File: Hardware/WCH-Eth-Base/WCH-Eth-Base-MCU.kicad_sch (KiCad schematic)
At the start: 47 parts, among them J1 Conn_02x03_Odd_Even, J2 Micro_SD_Card_Det1, J3 USB_C_Receptacle_USB2.0, J4 USB_C_Receptacle_USB2.0, SW1 SW_Push, SW2 SW_Push, U1 CH32V307VCT6, U2 WE-TVS-82400102, U3 WE-TVS-82400102, Y1 Crystal_GND24

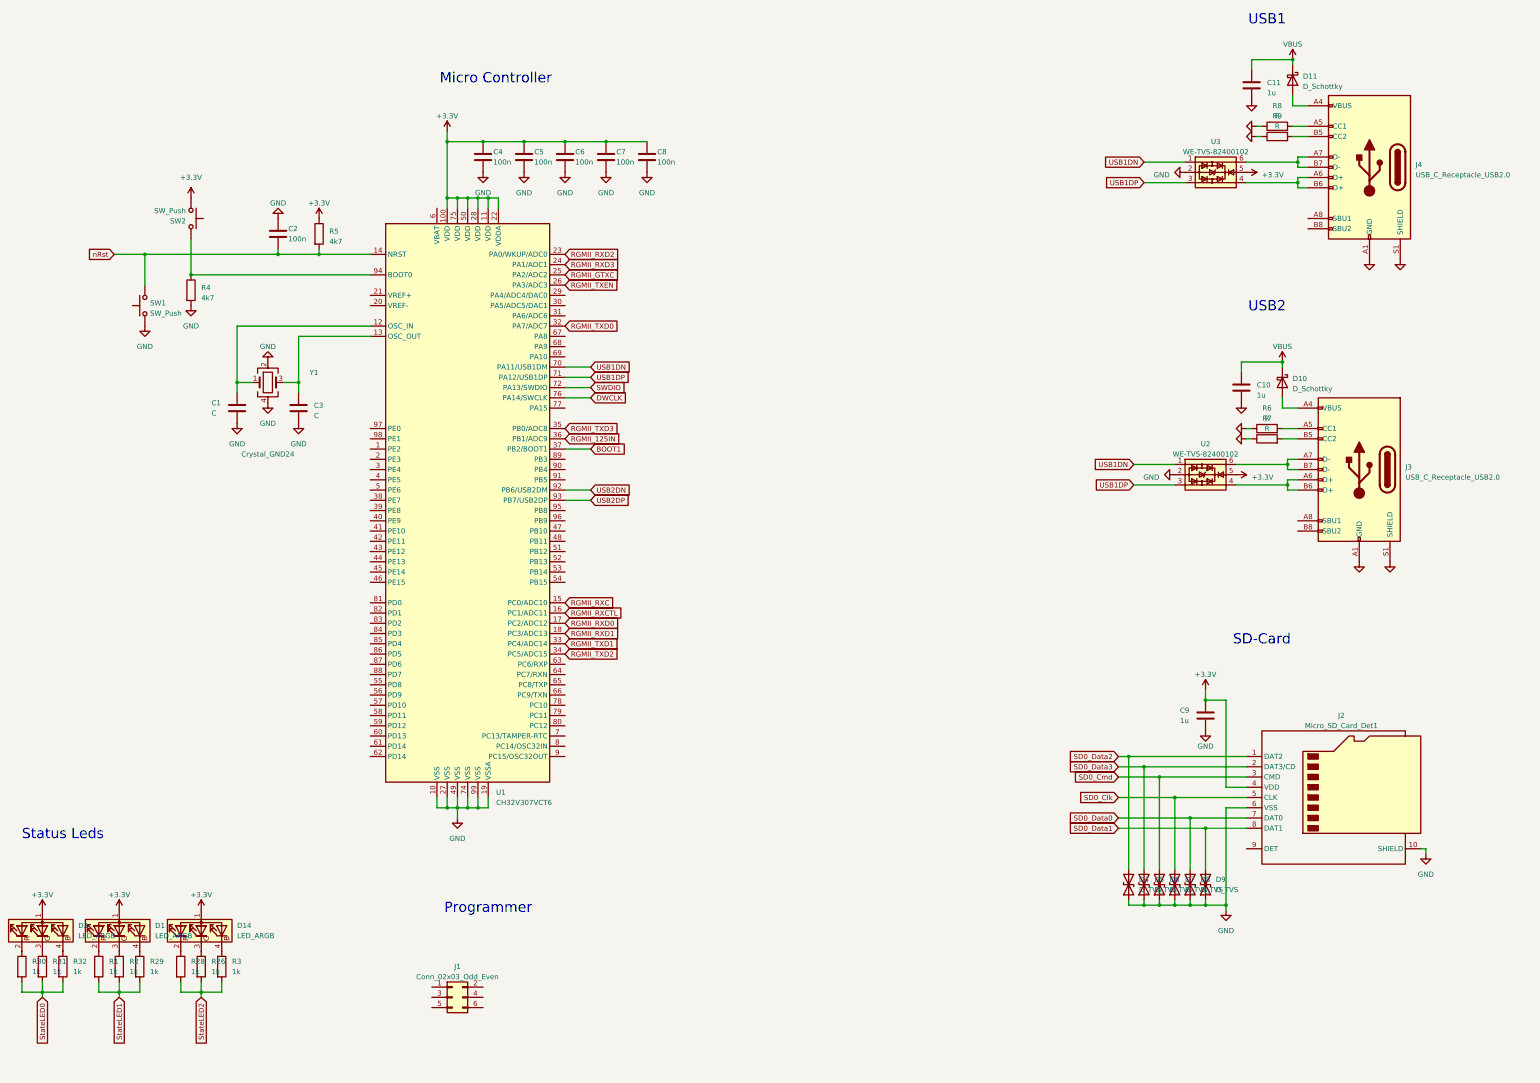
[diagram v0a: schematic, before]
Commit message: add Files and First Layout things
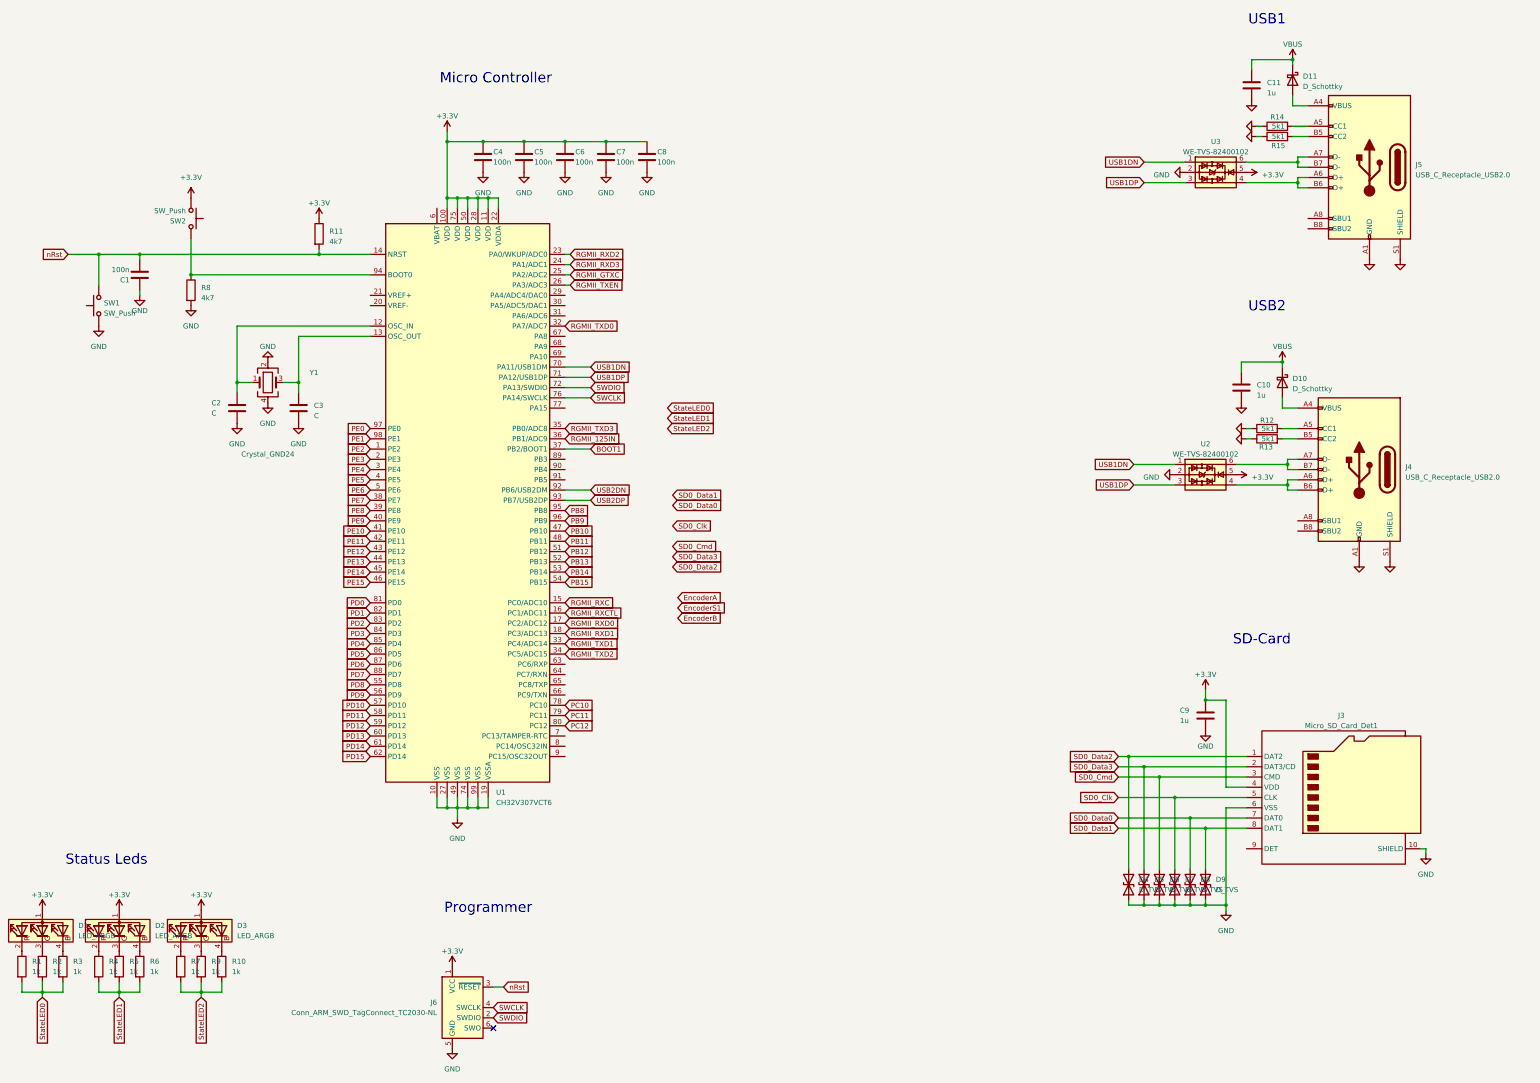
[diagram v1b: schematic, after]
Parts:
- removed J1: Conn_02x03_Odd_Even, symbol Connector_Generic:Conn_02x03_Odd_Even
- added J6: Conn_ARM_SWD_TagConnect_TC2030-NL, Connector:Tag-Connect_TC2030-IDC-NL_2x03_P1.27mm_Vertical, symbol Connector:Conn_ARM_SWD_TagConnect_TC2030-NL
- D10, D11, D4: footprint (none) -> Diode_SMD:D_SMA
- R12: renamed from R6; value R -> 5k1
- R13: renamed from R7; value R -> 5k1
- R14: renamed from R8; value R -> 5k1
- R15: renamed from R9; value R -> 5k1
- SW1, SW2: footprint (none) -> LCSC:SW-SMD_4P-L5.1-W5.1-P3.70-LS6.5-TL-2
- renumbered C2 to C1, C1 to C2, D2 to D1, D1 to D2, D14 to D3, J2 to J3, J3 to J4, J4 to J5, R30 to R1, R3 to R10, R5 to R11, R31 to R2, R32 to R3, R1 to R4, R2 to R5, R29 to R6, R28 to R7, R4 to R8, R26 to R9
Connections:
- net +3.3V: now also J6.1 (VCC)
- net GND: now also J6.5 (GND)
- net SWDIO: now also J6.2 (SWDIO)
- net nRst: now also J6.3 (~{RESET})
- net PE2: now reaches U1.1 (PE2)
- net PE3: now reaches U1.2 (PE3)
- net PE4: now reaches U1.3 (PE4)
- net PE7: now reaches U1.38 (PE7)
- net PE8: now reaches U1.39 (PE8)
- net PE5: now reaches U1.4 (PE5)
- net PE9: now reaches U1.40 (PE9)
- net PE10: now reaches U1.41 (PE10)
- net PE11: now reaches U1.42 (PE11)
- net PE12: now reaches U1.43 (PE12)
- net PE13: now reaches U1.44 (PE13)
- net PE14: now reaches U1.45 (PE14)
- net PE15: now reaches U1.46 (PE15)
- net PB10: now reaches U1.47 (PB10)
- net PB11: now reaches U1.48 (PB11)
- net PE6: now reaches U1.5 (PE6)
- net PB12: now reaches U1.51 (PB12)
- net PB13: now reaches U1.52 (PB13)
- net PB14: now reaches U1.53 (PB14)
- net PB15: now reaches U1.54 (PB15)
- net PD8: now reaches U1.55 (PD8)
- net PD9: now reaches U1.56 (PD9)
- net PD10: now reaches U1.57 (PD10)
- net PD11: now reaches U1.58 (PD11)
- net PD12: now reaches U1.59 (PD12)
- net PD13: now reaches U1.60 (PD13)
- net PD14: now reaches U1.61 (PD14)
- net PD15: now reaches U1.62 (PD14)
- net PC10: now reaches U1.78 (PC10)
- net PC11: now reaches U1.79 (PC11)
- net PC12: now reaches U1.80 (PC12)
- net PD0: now reaches U1.81 (PD0)
- net PD1: now reaches U1.82 (PD1)
- net PD2: now reaches U1.83 (PD2)
- net PD3: now reaches U1.84 (PD3)
- net PD4: now reaches U1.85 (PD4)
- net PD5: now reaches U1.86 (PD5)
- net PD6: now reaches U1.87 (PD6)
- net PD7: now reaches U1.88 (PD7)
- net PB8: now reaches U1.95 (PB8)
- net PB9: now reaches U1.96 (PB9)
- net PE0: now reaches U1.97 (PE0)
- net PE1: now reaches U1.98 (PE1)
- net DWCLK renamed SWCLK
- net SWCLK: now also J6.4 (SWCLK)
- no-connect marks 0 -> 1
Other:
- moved on the sheet: C1, SW1
